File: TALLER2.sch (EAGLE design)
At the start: 11 parts, among them IC1 LM741P, J2 1X5, K1 JJM1-12V, T1 2N2222

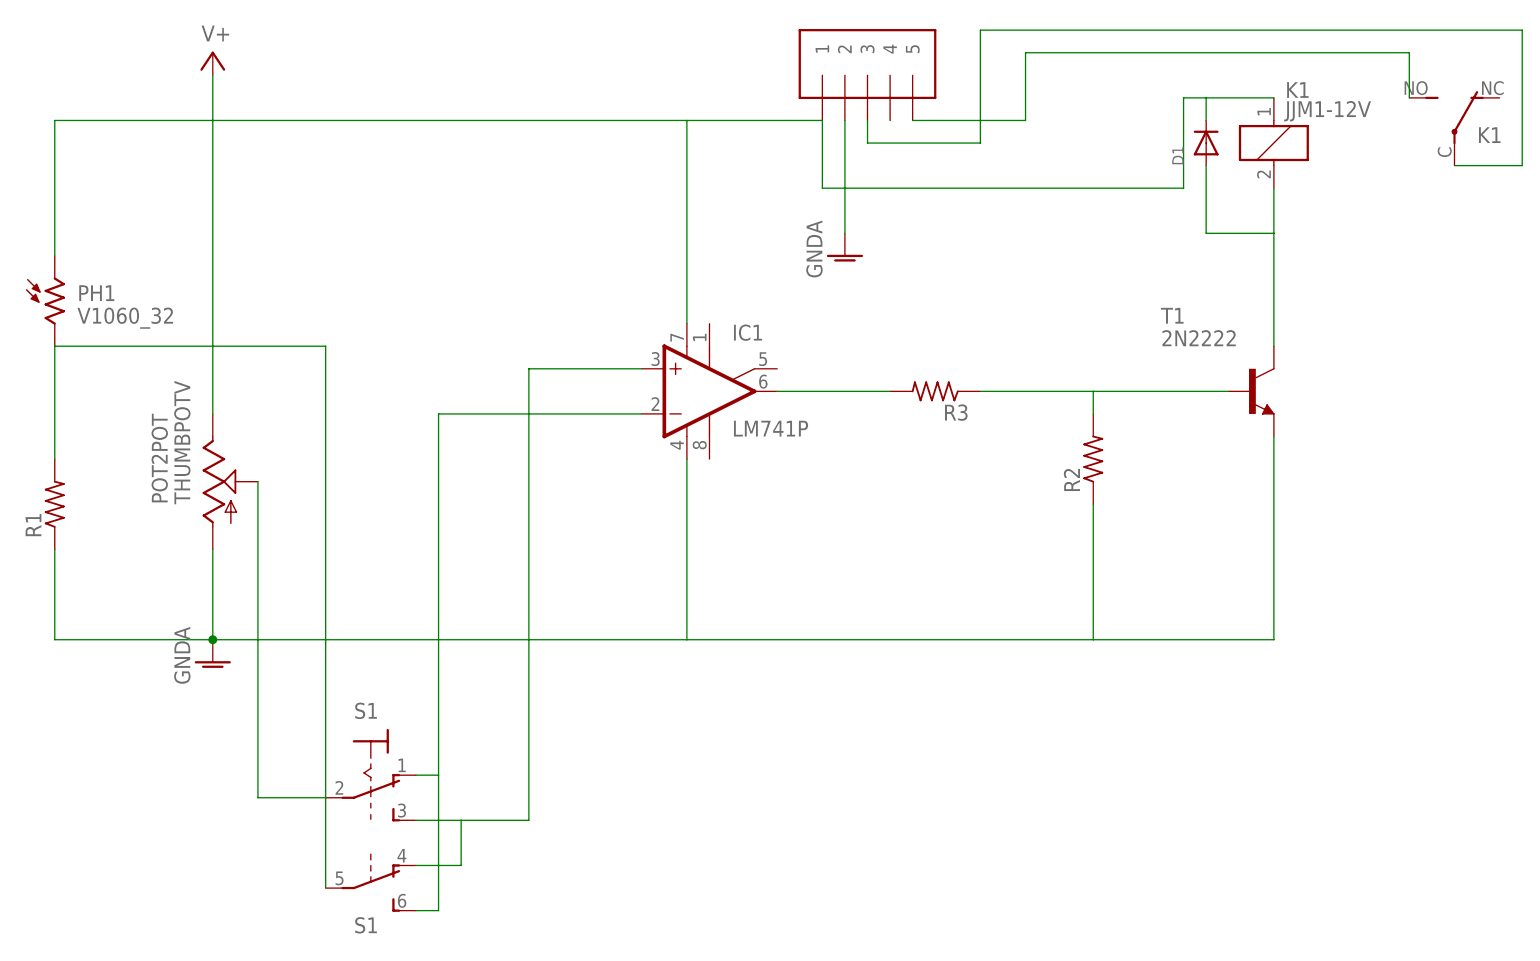
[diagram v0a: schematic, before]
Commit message: Final PCB
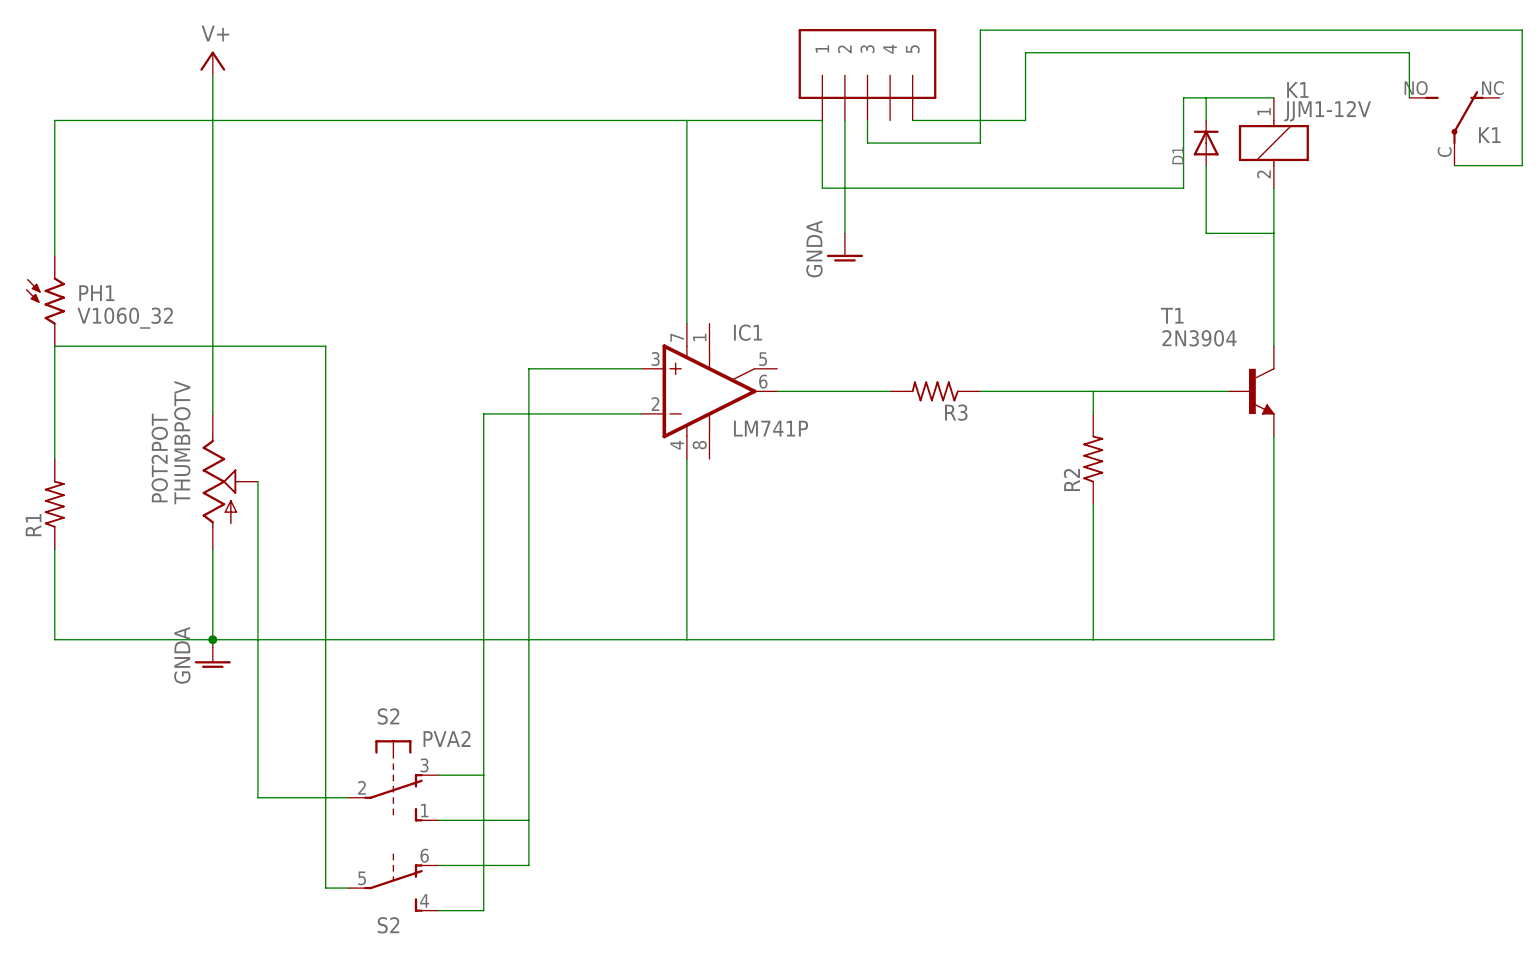
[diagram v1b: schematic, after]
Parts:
- removed S1: (no value), switch:320-938
- added S2: PVA2, switch-misc:PVA2
- T1: value 2N2222 -> 2N3904; device transistor-neu-to92:2N2222 -> transistor:2N3904
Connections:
- net N$2: now also S22.P; no longer S1B.P
- net N$4: now also S21.P; no longer S11.P
- net N$5: now also S21.O, S22.S; no longer S11.O, S1B.S
- net N$6: now also S21.S, S22.O; no longer S11.S, S1B.O
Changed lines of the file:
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@@
 <part name="R2" library="adafruit" deviceset="R-US_" device="0207/10"/>
 <part name="R3" library="adafruit" deviceset="R-US_" device="0207/10"/>
-<part name="T1" library="transistor-neu-to92" deviceset="2N2222" device=""/>
+<part name="T1" library="transistor" deviceset="2N3904" device=""/>
 <part name="K1" library="relay" deviceset="JJM1-12V" device=""/>
 <part name="PH1" library="photo-elements" deviceset="?1060*" device="V" technology="_32"/>
@@
 <part name="SUPPLY1" library="supply2" deviceset="V+" device=""/>
 <part name="GND1" library="supply1" deviceset="GNDA" device=""/>
-<part name="S1" library="switch" deviceset="320-938" device=""/>
 <part name="D1" library="adafruit" deviceset="DIODE" device="DO-1N4148"/>
 <part name="GND2" library="supply1" deviceset="GNDA" device=""/>
+<part name="S2" library="switch-misc" deviceset="PVA2" device=""/>
 </parts>
 <sheets>
@@
 <instance part="R2" gate="G$1" x="96.52" y="45.72" rot="R90"/>
 <instance part="R3" gate="G$1" x="78.74" y="53.34" rot="R180"/>
-<instance part="T1" gate="G$1" x="114.3" y="53.34"/>
+<instance part="T1" gate="G1" x="114.3" y="53.34"/>
 <instance part="K1" gate="1" x="116.84" y="81.28"/>
 <instance part="K1" gate="2" x="137.16" y="81.28"/>
@@
 <instance part="SUPPLY1" gate="1" x="-2.54" y="91.44"/>
 <instance part="GND1" gate="1" x="-2.54" y="22.86"/>
-<instance part="S1" gate="B" x="15.24" y="-2.54" rot="R270"/>
-<instance part="S1" gate="1" x="15.24" y="10.16" rot="R270"/>
 <instance part="D1" gate="G$1" x="109.22" y="81.28" rot="R90"/>
 <instance part="GND2" gate="1" x="68.58" y="68.58"/>
+<instance part="S2" gate="1" x="17.78" y="7.62" rot="R270"/>
+<instance part="S2" gate="2" x="17.78" y="-2.54" rot="R270"/>
 </instances>
 <busses>
@@
 <pinref part="PH1" gate="G$1" pin="2"/>
 <wire x1="-20.32" y1="45.72" x2="-20.32" y2="58.42" width="0.1524" layer="91"/>
-<pinref part="S1" gate="B" pin="P"/>
 <wire x1="-20.32" y1="58.42" x2="10.16" y2="58.42" width="0.1524" layer="91"/>
 <wire x1="10.16" y1="58.42" x2="10.16" y2="-2.54" width="0.1524" layer="91"/>
+<pinref part="S2" gate="2" pin="P"/>
+<wire x1="10.16" y1="-2.54" x2="12.7" y2="-2.54" width="0.1524" layer="91"/>
 </segment>
 </net>
@@
 <wire x1="50.8" y1="25.4" x2="96.52" y2="25.4" width="0.1524" layer="91"/>
 <wire x1="96.52" y1="25.4" x2="96.52" y2="40.64" width="0.1524" layer="91"/>
-<pinref part="T1" gate="G$1" pin="E"/>
+<pinref part="T1" gate="G1" pin="E"/>
 <wire x1="116.84" y1="48.26" x2="116.84" y2="25.4" width="0.1524" layer="91"/>
 <wire x1="116.84" y1="25.4" x2="96.52" y2="25.4" width="0.1524" layer="91"/>
@@
 <net name="N$4" class="0">
 <segment>
-<pinref part="S1" gate="1" pin="P"/>
 <pinref part="POT2" gate="POT" pin="S"/>
-<wire x1="10.16" y1="7.62" x2="2.54" y2="7.62" width="0.1524" layer="91"/>
 <wire x1="2.54" y1="7.62" x2="2.54" y2="43.18" width="0.1524" layer="91"/>
+<pinref part="S2" gate="1" pin="P"/>
+<wire x1="12.7" y1="7.62" x2="2.54" y2="7.62" width="0.1524" layer="91"/>
 </segment>
 </net>
 <net name="N$5" class="0">
 <segment>
-<pinref part="S1" gate="1" pin="O"/>
-<wire x1="20.32" y1="10.16" x2="22.86" y2="10.16" width="0.1524" layer="91"/>
-<wire x1="22.86" y1="10.16" x2="22.86" y2="50.8" width="0.1524" layer="91"/>
 <pinref part="IC1" gate="A" pin="-IN"/>
-<wire x1="22.86" y1="50.8" x2="45.72" y2="50.8" width="0.1524" layer="91"/>
-<pinref part="S1" gate="B" pin="S"/>
-<wire x1="20.32" y1="-5.08" x2="22.86" y2="-5.08" width="0.1524" layer="91"/>
-<wire x1="22.86" y1="-5.08" x2="22.86" y2="10.16" width="0.1524" layer="91"/>
+<wire x1="27.94" y1="10.16" x2="27.94" y2="50.8" width="0.1524" layer="91"/>
+<wire x1="27.94" y1="50.8" x2="45.72" y2="50.8" width="0.1524" layer="91"/>
+<pinref part="S2" gate="2" pin="S"/>
+<wire x1="22.86" y1="-5.08" x2="27.94" y2="-5.08" width="0.1524" layer="91"/>
+<wire x1="27.94" y1="-5.08" x2="27.94" y2="10.16" width="0.1524" layer="91"/>
+<pinref part="S2" gate="1" pin="O"/>
+<wire x1="22.86" y1="10.16" x2="27.94" y2="10.16" width="0.1524" layer="91"/>
 </segment>
 </net>
 <net name="N$6" class="0">
 <segment>
-<pinref part="S1" gate="B" pin="O"/>
-<wire x1="20.32" y1="0" x2="25.4" y2="0" width="0.1524" layer="91"/>
-<wire x1="25.4" y1="0" x2="25.4" y2="5.08" width="0.1524" layer="91"/>
-<wire x1="25.4" y1="5.08" x2="33.02" y2="5.08" width="0.1524" layer="91"/>
+<pinref part="IC1" gate="A" pin="+IN"/>
 <wire x1="33.02" y1="5.08" x2="33.02" y2="55.88" width="0.1524" layer="91"/>
-<pinref part="IC1" gate="A" pin="+IN"/>
 <wire x1="33.02" y1="55.88" x2="45.72" y2="55.88" width="0.1524" layer="91"/>
-<pinref part="S1" gate="1" pin="S"/>
-<wire x1="20.32" y1="5.08" x2="25.4" y2="5.08" width="0.1524" layer="91"/>
+<pinref part="S2" gate="2" pin="O"/>
+<wire x1="22.86" y1="0" x2="33.02" y2="0" width="0.1524" layer="91"/>
+<wire x1="33.02" y1="0" x2="33.02" y2="5.08" width="0.1524" layer="91"/>
+<pinref part="S2" gate="1" pin="S"/>
+<wire x1="22.86" y1="5.08" x2="33.02" y2="5.08" width="0.1524" layer="91"/>
 </segment>
 </net>
@@
 <wire x1="83.82" y1="53.34" x2="96.52" y2="53.34" width="0.1524" layer="91"/>
 <wire x1="96.52" y1="53.34" x2="96.52" y2="50.8" width="0.1524" layer="91"/>
-<pinref part="T1" gate="G$1" pin="B"/>
+<pinref part="T1" gate="G1" pin="B"/>
 <wire x1="111.76" y1="53.34" x2="96.52" y2="53.34" width="0.1524" layer="91"/>
 </segment>
@@
 <net name="N$9" class="0">
 <segment>
-<pinref part="T1" gate="G$1" pin="C"/>
+<pinref part="T1" gate="G1" pin="C"/>
 <pinref part="K1" gate="1" pin="2"/>
 <wire x1="116.84" y1="58.42" x2="116.84" y2="71.12" width="0.1524" layer="91"/>
